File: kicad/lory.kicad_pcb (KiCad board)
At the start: 2 copper layers, 123.5 x 85.3 mm, 48 parts, among them J1 MJ-4PP-9, SW10 SW_PUSH, SW11 SW_PUSH, SW12 SW_PUSH, SW14 SW_PUSH, SW15 SW_PUSH, SW16 SW_PUSH, SW17 SW_PUSH, SW18 SW_PUSH, SW2 SW_PUSH, SW20 SW_PUSH, SW21 SW_PUSH, SW3 SW_PUSH, SW4 SW_PUSH, SW5 SW_PUSH, SW6 SW_PUSH, SW8 SW_PUSH, SW9 SW_PUSH, U1 ProMicro

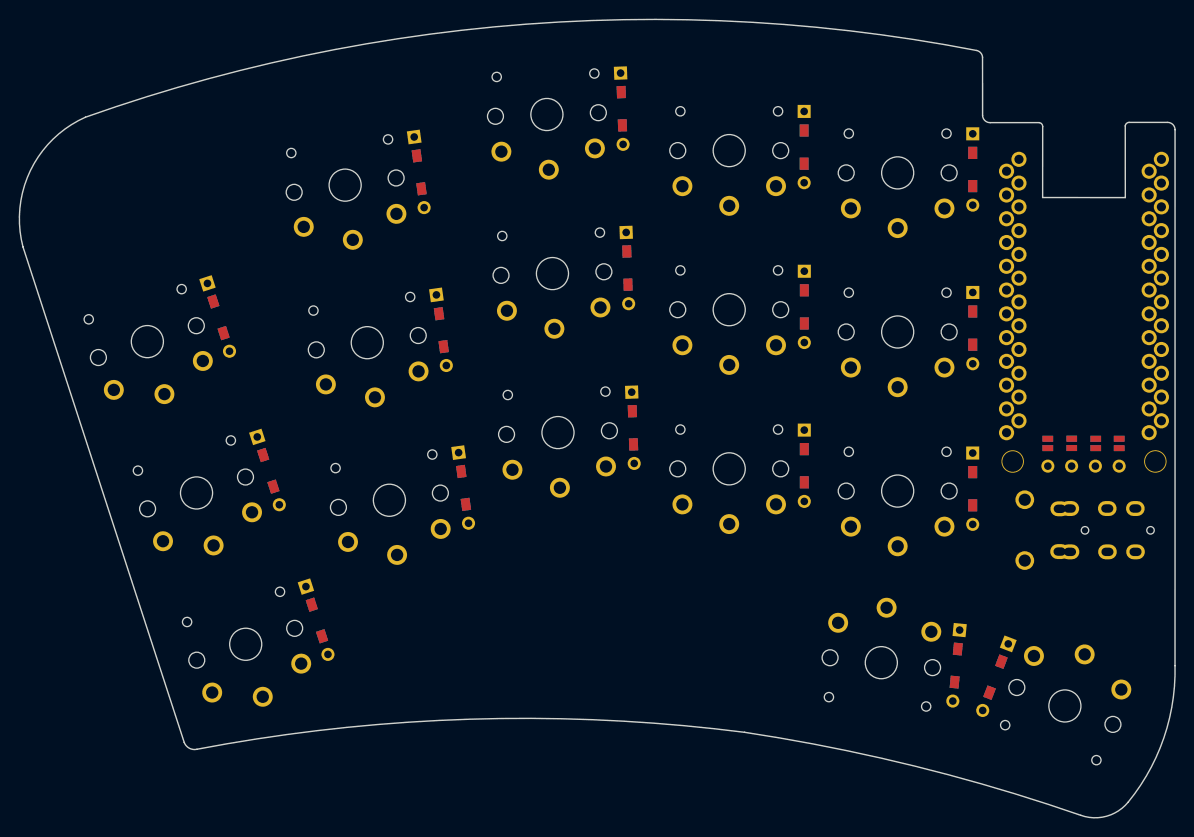
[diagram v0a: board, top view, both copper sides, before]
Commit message: temp
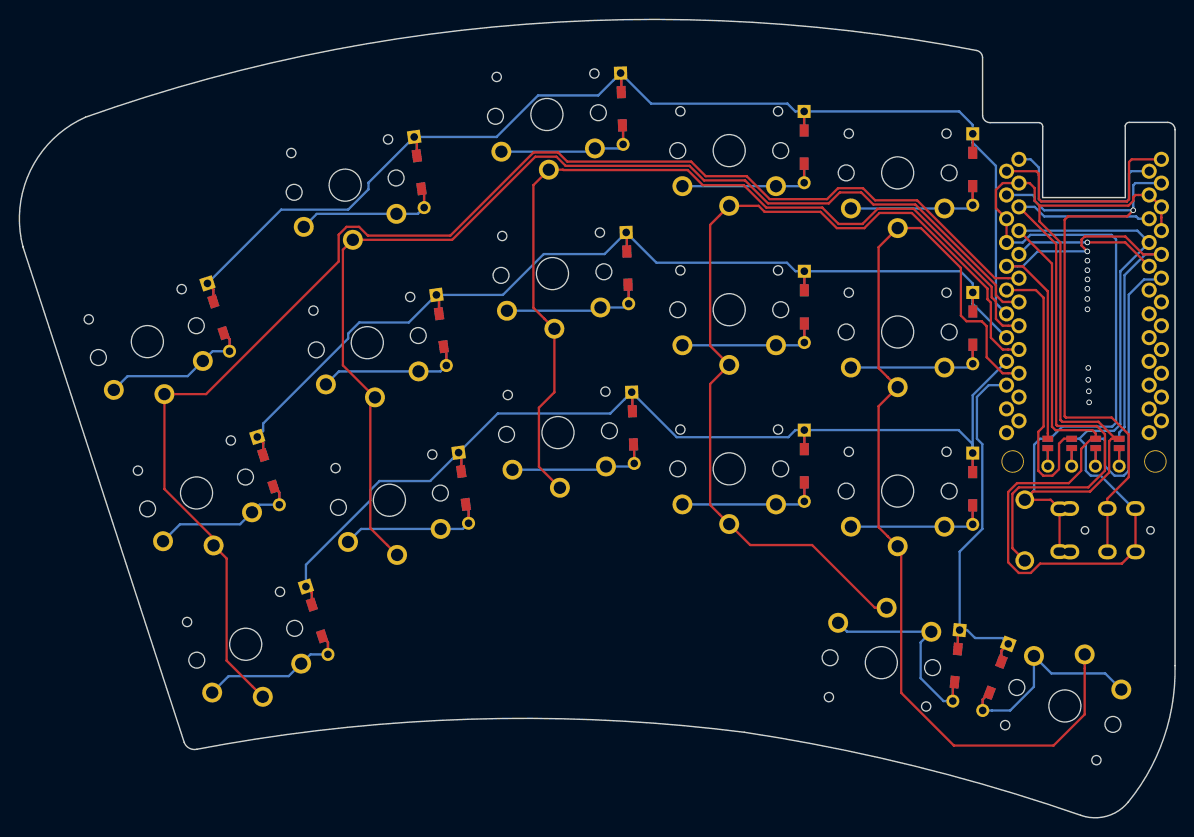
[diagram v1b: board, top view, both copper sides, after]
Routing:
- net col1: track 0.00 -> 147.7 mm, vias 0 -> 1
- net row0: track 0.00 -> 136.4 mm, vias 0 -> 1
- net GND: track 0.00 -> 134.4 mm
- net col2: track 0.00 -> 120.5 mm, vias 0 -> 1
- net VCC: track 0.00 -> 119.8 mm
- net row2: track 0.00 -> 118.0 mm
- net row1: track 0.00 -> 116.7 mm, vias 0 -> 1
- net col5: track 0.00 -> 107.2 mm
- net col4: track 0.00 -> 99.4 mm
- net col3: track 0.00 -> 97.8 mm, vias 0 -> 1
- net data: track 0.00 -> 70.2 mm, vias 0 -> 1
- net reset: track 0.00 -> 67.5 mm
- net SDA: track 0.00 -> 64.1 mm, vias 0 -> 1
- net SCL: track 0.00 -> 60.1 mm, vias 0 -> 1
- net row3: track 0.00 -> 44.3 mm
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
